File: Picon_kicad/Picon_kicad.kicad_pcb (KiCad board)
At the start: 2 copper layers, 86.9 x 46.9 mm, 0 parts

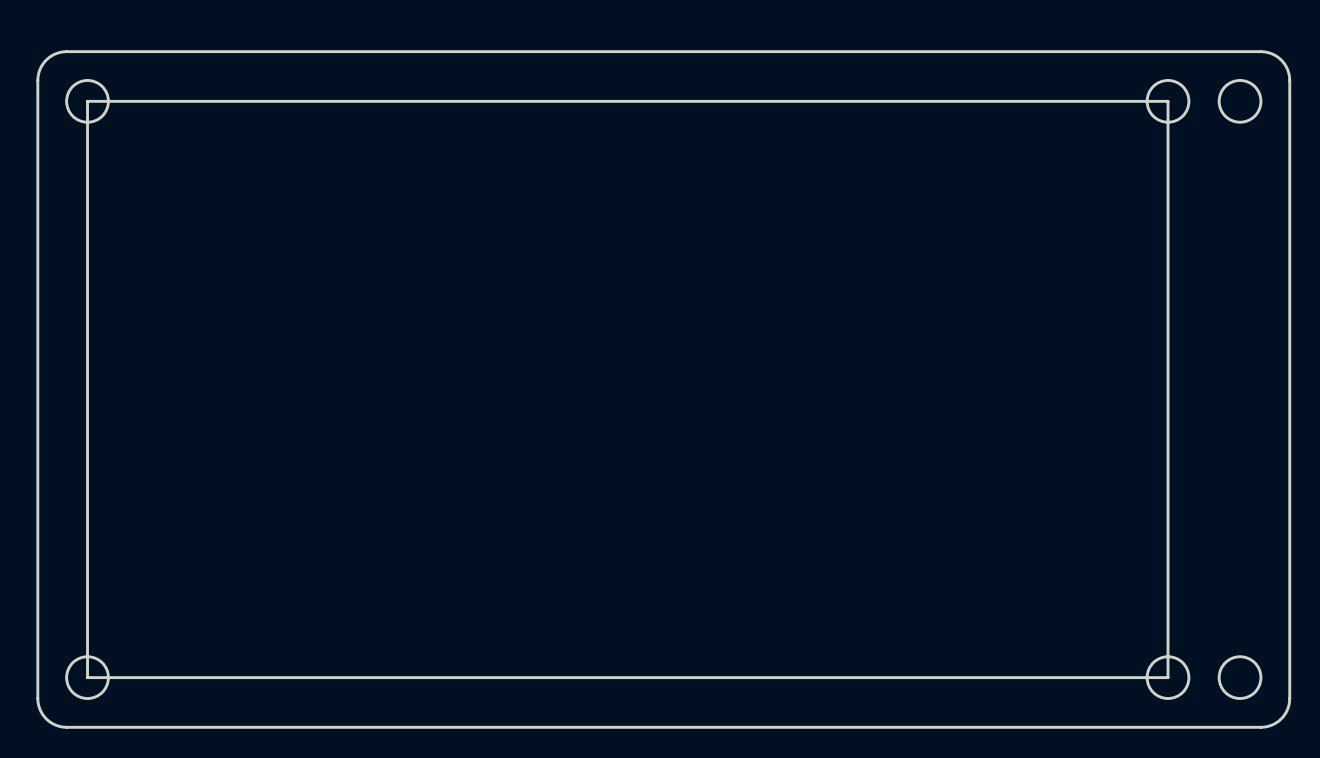
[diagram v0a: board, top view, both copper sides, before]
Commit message: v0.2 | Rudimentary PCB layout
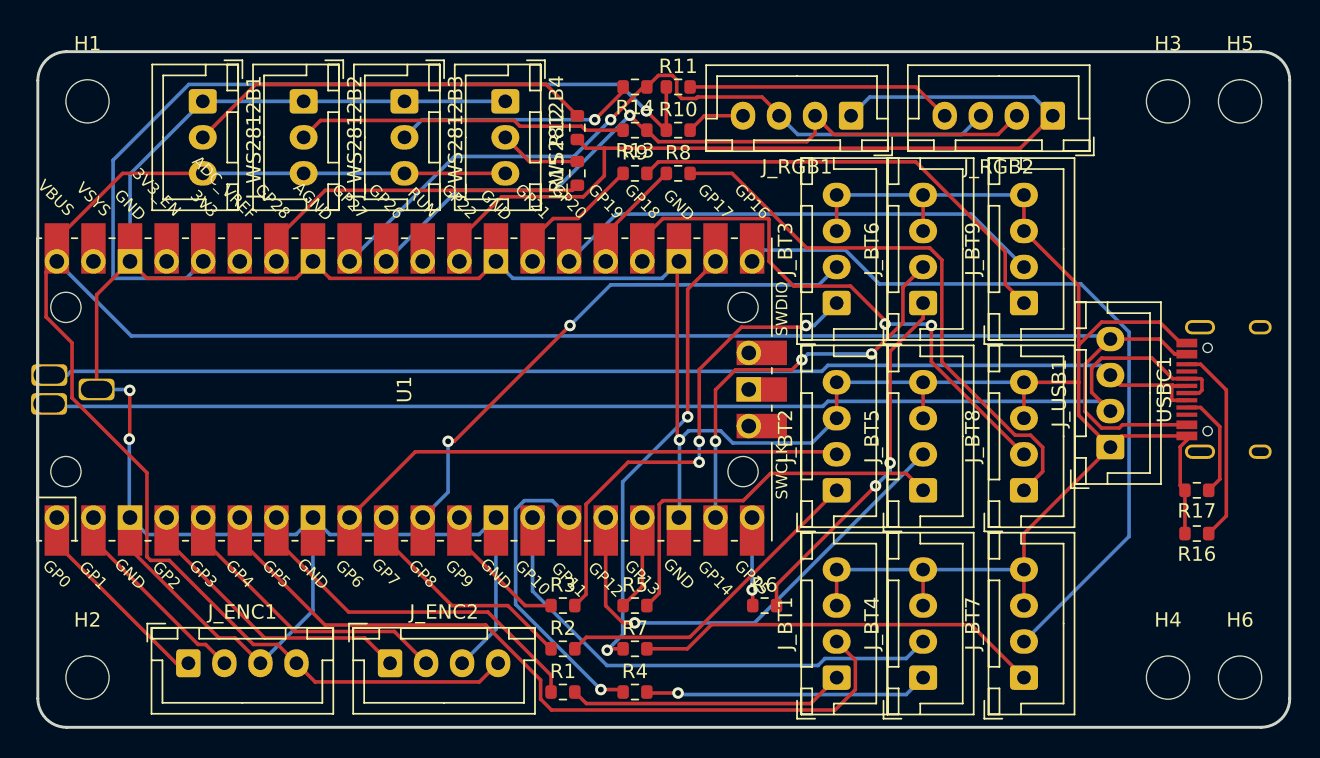
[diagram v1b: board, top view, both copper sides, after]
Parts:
- added H1: MountingHole, MountingHole:MountingHole_3mm, F.Cu at (110.0, 85.0)
- added H2: MountingHole, MountingHole:MountingHole_3mm, F.Cu at (110.0, 125.0)
- added H3: MountingHole, MountingHole:MountingHole_3mm, F.Cu at (185.0, 85.0)
- added H4: MountingHole, MountingHole:MountingHole_3mm, F.Cu at (185.0, 125.0)
- added H5: MountingHole, MountingHole:MountingHole_3mm, F.Cu at (190.0, 85.0)
- added H6: MountingHole, MountingHole:MountingHole_3mm, F.Cu at (190.0, 125.0)
- added J_BT1: Conn_01x04, Connector_JST:JST_XH_B4B-XH-A_1x04_P2.50mm_Vertical, F.Cu at (162.0, 125.0)
- added J_BT2: Conn_01x04, Connector_JST:JST_XH_B4B-XH-A_1x04_P2.50mm_Vertical, F.Cu at (162.0, 112.0)
- added J_BT3: Conn_01x04, Connector_JST:JST_XH_B4B-XH-A_1x04_P2.50mm_Vertical, F.Cu at (162.0, 99.0)
- added J_BT4: Conn_01x04, Connector_JST:JST_XH_B4B-XH-A_1x04_P2.50mm_Vertical, F.Cu at (168.0, 125.0)
- added J_BT5: Conn_01x04, Connector_JST:JST_XH_B4B-XH-A_1x04_P2.50mm_Vertical, F.Cu at (168.0, 112.0)
- added J_BT6: Conn_01x04, Connector_JST:JST_XH_B4B-XH-A_1x04_P2.50mm_Vertical, F.Cu at (168.0, 99.0)
- added J_BT7: Conn_01x04, Connector_JST:JST_XH_B4B-XH-A_1x04_P2.50mm_Vertical, F.Cu at (175.0, 125.0)
- added J_BT8: Conn_01x04, Connector_JST:JST_XH_B4B-XH-A_1x04_P2.50mm_Vertical, F.Cu at (175.0, 112.0)
- added J_BT9: Conn_01x04, Connector_JST:JST_XH_B4B-XH-A_1x04_P2.50mm_Vertical, F.Cu at (175.0, 99.0)
- added J_ENC1: Conn_01x04, Connector_JST:JST_XH_B4B-XH-A_1x04_P2.50mm_Vertical, F.Cu at (117.0, 124.0)
- added J_ENC2: Conn_01x04, Connector_JST:JST_XH_B4B-XH-A_1x04_P2.50mm_Vertical, F.Cu at (131.0, 124.0)
- added J_RGB1: Conn_01x04, Connector_JST:JST_XH_B4B-XH-A_1x04_P2.50mm_Vertical, F.Cu at (163.0, 86.0)
- added J_RGB2: Conn_01x04, Connector_JST:JST_XH_B4B-XH-A_1x04_P2.50mm_Vertical, F.Cu at (177.0, 86.0)
- added J_USB1: Conn_01x04, Connector_JST:JST_XH_B4B-XH-A_1x04_P2.50mm_Vertical, F.Cu at (181.0, 109.0)
- added J_WS2812B1: Conn_01x03, Connector_JST:JST_XH_B3B-XH-A_1x03_P2.50mm_Vertical, F.Cu at (118.0, 85.0)
- added J_WS2812B2: Conn_01x03, Connector_JST:JST_XH_B3B-XH-A_1x03_P2.50mm_Vertical, F.Cu at (125.0, 85.0)
- added J_WS2812B3: Conn_01x03, Connector_JST:JST_XH_B3B-XH-A_1x03_P2.50mm_Vertical, F.Cu at (132.0, 85.0)
- added J_WS2812B4: Conn_01x03, Connector_JST:JST_XH_B3B-XH-A_1x03_P2.50mm_Vertical, F.Cu at (139.0, 85.0)
- added R1: 120R, Resistor_SMD:R_0603_1608Metric, F.Cu at (143.0, 126.0)
- added R10: 120R, Resistor_SMD:R_0603_1608Metric, F.Cu at (151.0, 87.0)
- added R11: 120R, Resistor_SMD:R_0603_1608Metric, F.Cu at (151.0, 84.0)
- added R12: 120R, Resistor_SMD:R_0603_1608Metric, F.Cu at (144.0, 86.8)
- added R13: 120R, Resistor_SMD:R_0603_1608Metric, F.Cu at (148.0, 87.0)
- added R14: 120R, Resistor_SMD:R_0603_1608Metric, F.Cu at (148.0, 84.0)
- added R15: 120R, Resistor_SMD:R_0603_1608Metric, F.Cu at (144.0, 90.0)
- added R16: 5K1, Resistor_SMD:R_0603_1608Metric, F.Cu at (187.0, 115.0)
- added R17: 5K1, Resistor_SMD:R_0603_1608Metric, F.Cu at (187.0, 112.0)
- added R2: 120R, Resistor_SMD:R_0603_1608Metric, F.Cu at (143.0, 123.0)
- added R3: 120R, Resistor_SMD:R_0603_1608Metric, F.Cu at (143.0, 120.0)
- added R4: 120R, Resistor_SMD:R_0603_1608Metric, F.Cu at (148.0, 126.0)
- added R5: 120R, Resistor_SMD:R_0603_1608Metric, F.Cu at (148.0, 120.0)
- added R6: 120R, Resistor_SMD:R_0603_1608Metric, F.Cu at (157.0, 120.0)
- added R7: 120R, Resistor_SMD:R_0603_1608Metric, F.Cu at (148.0, 123.0)
- added R8: 120R, Resistor_SMD:R_0603_1608Metric, F.Cu at (151.0, 90.0)
- added R9: 120R, Resistor_SMD:R_0603_1608Metric, F.Cu at (148.0, 90.0)
- added U1: Pico, MCU_RaspberryPi_and_Boards:RPi_Pico_SMD_TH, F.Cu at (132.0, 105.0)
- added USBC1: HRO-TYPE-C-31-M-12, Type-C:HRO-TYPE-C-31-M-12-Assembly, F.Cu at (194.0, 105.0)
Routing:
- net GND: track 0.00 -> 306.2 mm, vias 0 -> 3
- net VBUS: track 0.00 -> 181.3 mm
- net /USB_DP: track 0.00 -> 88.1 mm
- net /USB_DN: track 0.00 -> 82.8 mm
- net /RGB1: track 0.00 -> 64.6 mm
- net +3V3: track 0.00 -> 59.8 mm, vias 0 -> 1
- net /BT1: track 0.00 -> 54.4 mm
- net /BT7: track 0.00 -> 53.4 mm
- net /RGB3: track 0.00 -> 52.1 mm, vias 0 -> 1
- net /RGB2: track 0.00 -> 51.3 mm, vias 0 -> 1
- net Net-(J_BT8-Pad1): track 0.00 -> 40.0 mm
- net /BT8: track 0.00 -> 38.7 mm, vias 0 -> 2
- net /BT3: track 0.00 -> 38.0 mm, vias 0 -> 2
- net /BT2: track 0.00 -> 35.8 mm
- net /BT4: track 0.00 -> 35.0 mm
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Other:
- outline, holes or cut-outs redrawn
- net class Power added: clearance 0.2, trace_width 0.25, via_dia 0.8, via_drill 0.4
